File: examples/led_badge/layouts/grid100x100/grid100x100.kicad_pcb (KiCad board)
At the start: 4 copper layers, 200 parts

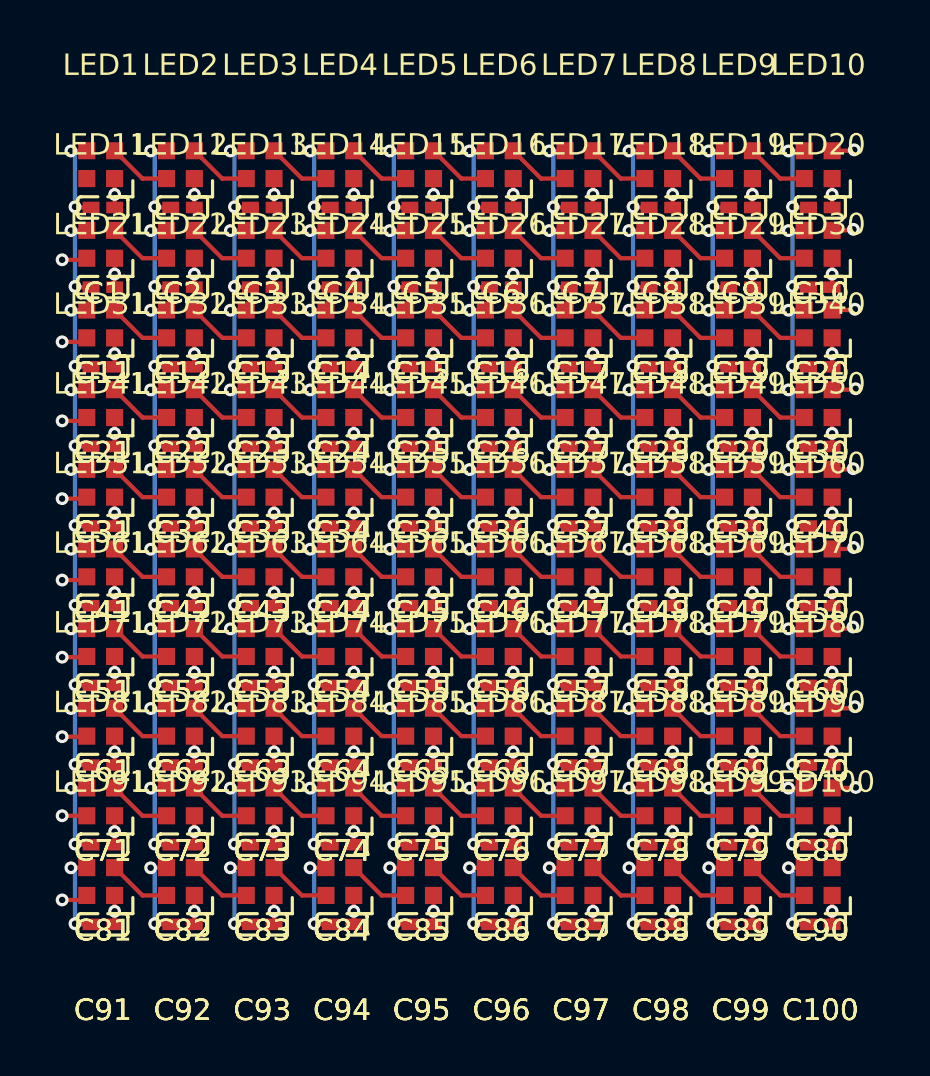
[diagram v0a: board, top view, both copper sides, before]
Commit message: almost complete layout
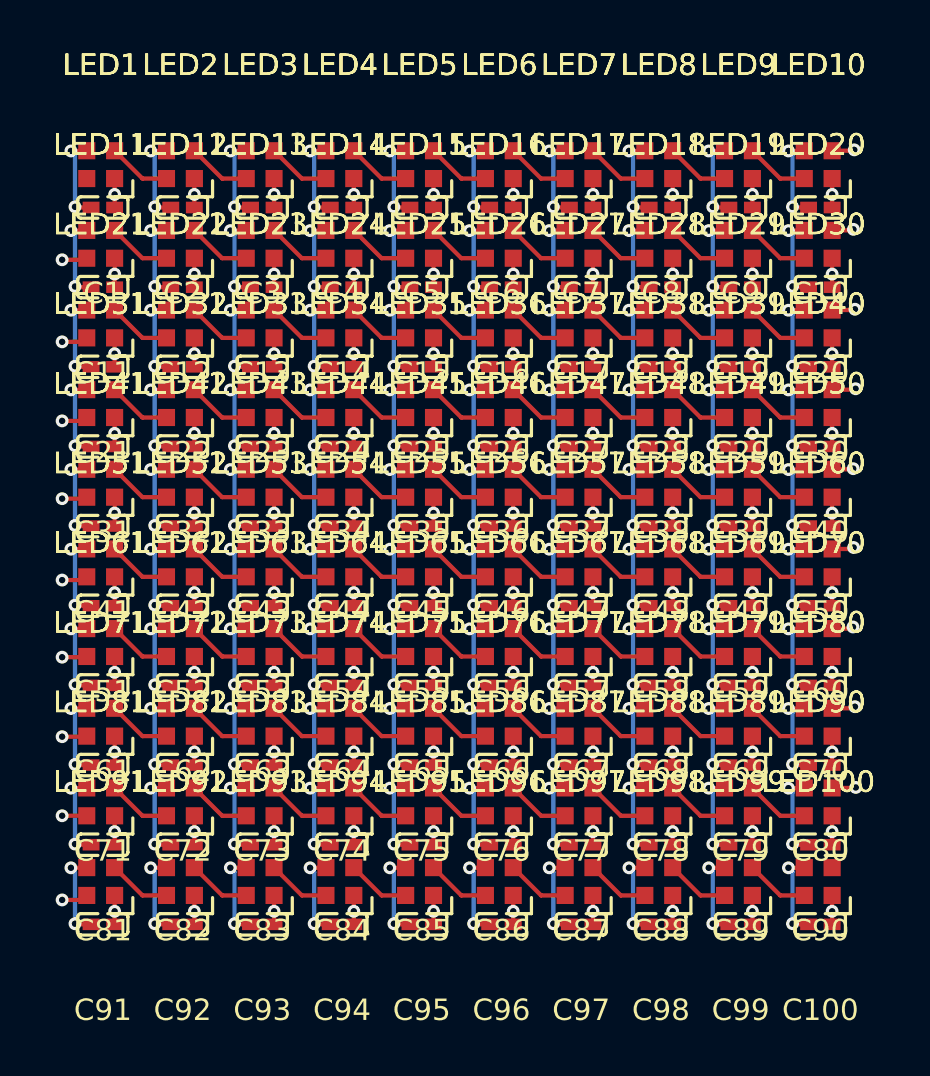
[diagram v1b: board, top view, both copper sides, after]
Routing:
- net hv: track 135.0 -> 173.8 mm
